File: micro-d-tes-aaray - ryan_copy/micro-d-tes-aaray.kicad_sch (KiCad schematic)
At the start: 46 parts, among them J1 Conn_01x01_Socket, J10 Conn_01x01_Socket, J11 Conn_01x01_Socket, J12 Conn_01x01_Socket, J13 Conn_01x01_Socket, J14 Conn_01x01_Socket, J15 Conn_01x01_Socket, J16 Conn_01x01_Socket, J17 Conn_01x01_Socket, J18 Conn_01x01_Socket, J2 Conn_01x01_Socket, J20 Conn_01x01_Socket, J21 DB25_Plug, J22 Conn_01x01_Socket, J23 Conn_01x01_Socket, J24 Conn_01x01_Socket, J25 Conn_01x01_Socket, J26 Conn_01x01_Socket, J27 Conn_01x01_Socket, J28 Conn_01x01_Socket, J29 Conn_01x01_Socket, J3 Conn_01x01_Socket, J30 Conn_01x01_Socket, J31 Conn_01x01_Socket, J32 Conn_01x01_Socket, J33 Conn_01x01_Socket, J34 Conn_01x01_Socket, J35 Conn_01x01_Socket, J36 Conn_01x01_Socket, J37 Conn_01x01_Socket, J38 Conn_01x01_Socket, J39 Conn_01x01_Socket, J4 Conn_01x01_Socket, J40 Conn_01x01_Socket, J41 Conn_01x01_Socket, J42 DB25_Plug, J5 Conn_01x01_Socket, J6 Conn_01x01_Socket, J7 Conn_01x01_Socket, J8 Conn_01x01_Socket, J9 Conn_01x01_Socket

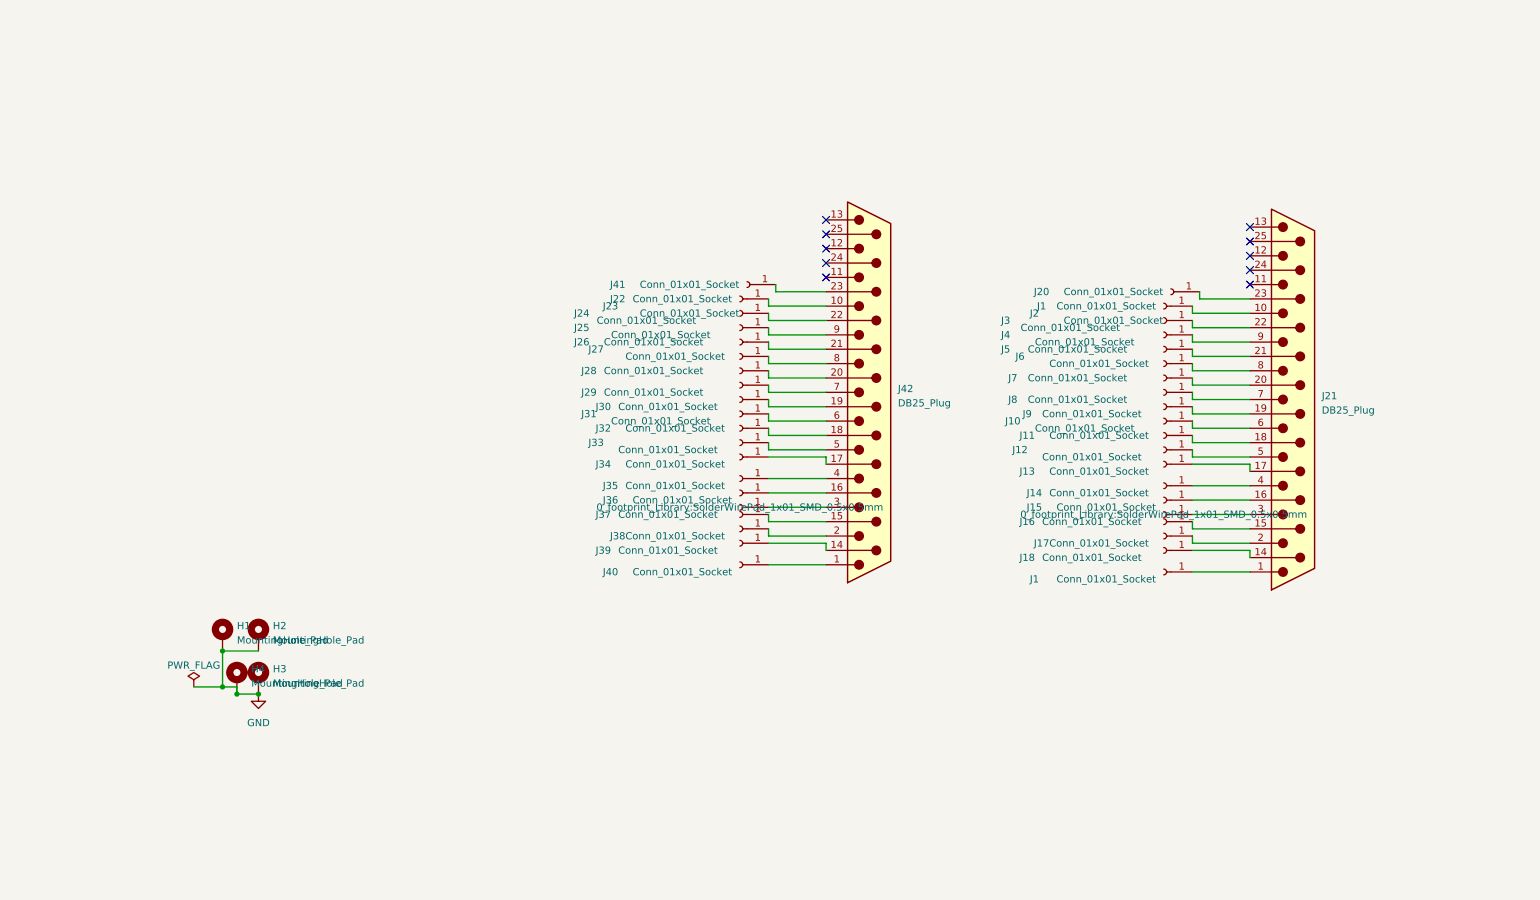
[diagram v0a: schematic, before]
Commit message: update
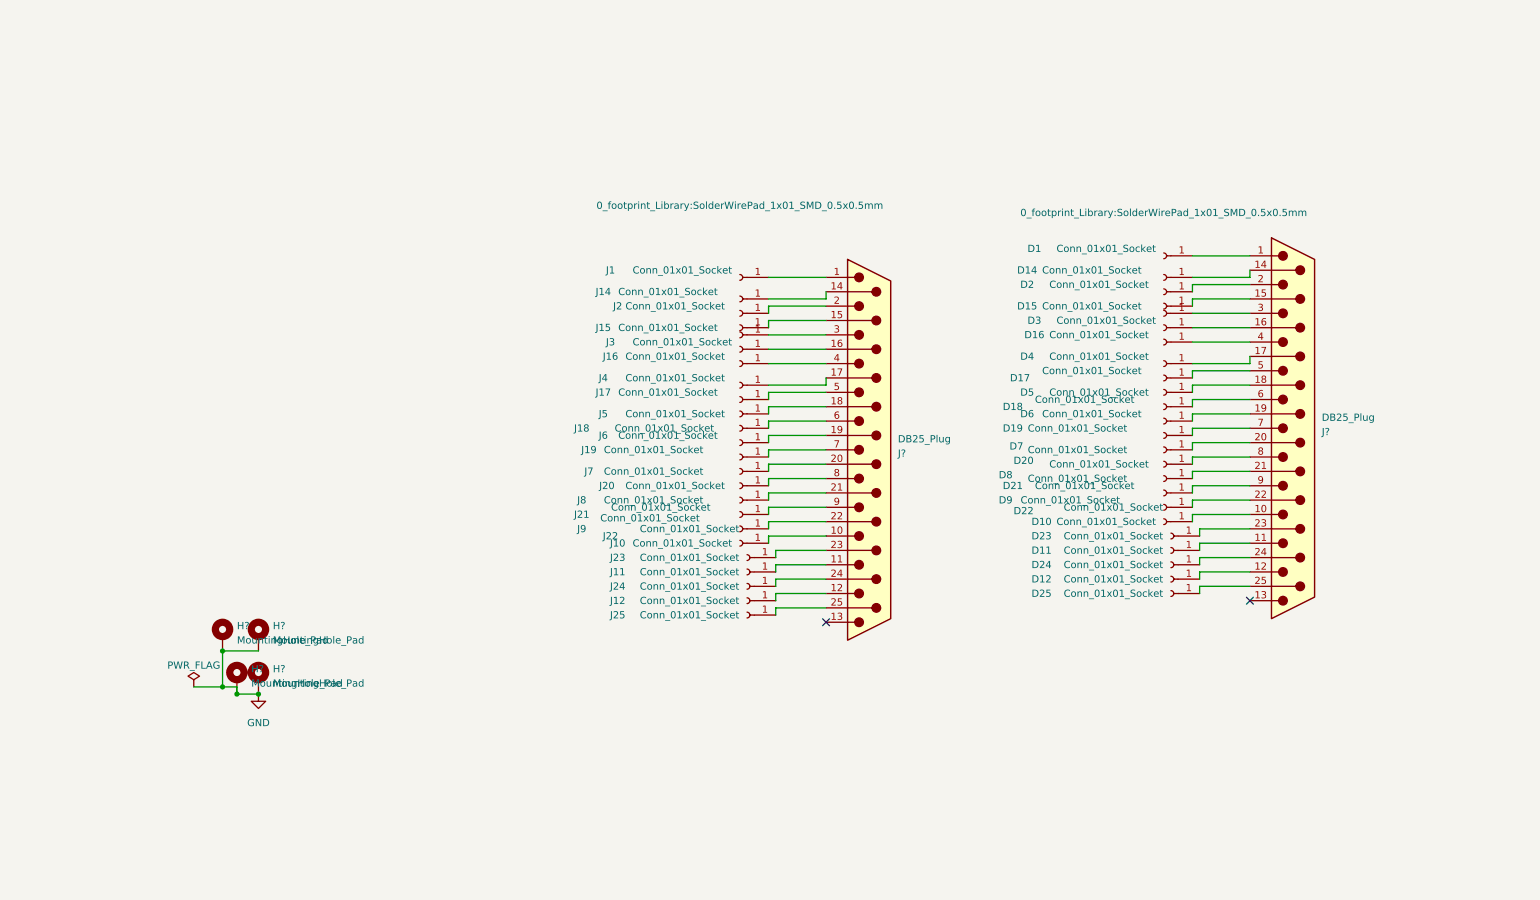
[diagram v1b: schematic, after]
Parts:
- added D11, D12, D24, D25, J11, J12, J24, J25: Conn_01x01_Socket, 0_footprint_Library:SolderWirePad_1x01_SMD_0.5x0.5mm, symbol Connector:Conn_01x01_Socket
- renumbered J1 to D1, J1 to D10, J18 to D14, J16 to D15, J14 to D16, J12 to D17, J10 to D18, J8 to D19, J17 to D2, J6 to D20, J4 to D21, J2 to D22, J20 to D23, J15 to D3, J13 to D4, J11 to D5, J9 to D6, J7 to D7, J5 to D8, J3 to D9, H4 to H?, H1 to H?, H2 to H?, H3 to H?, J40 to J1, J22 to J10, J39 to J14, J37 to J15, J35 to J16, J33 to J17, J31 to J18, J29 to J19, J38 to J2, J27 to J20, J25 to J21, J23 to J22, J41 to J23, J36 to J3, J34 to J4, J32 to J5, J30 to J6, J28 to J7, J26 to J8, J24 to J9, J42 to J?, J21 to J?
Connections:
- net at J?.11: now also J11.1 (Pin_1)
- net at J?.12: now also J12.1 (Pin_1)
- net at J?.24 (P24): now also J24.1 (Pin_1)
- net at J?.25 (P25): now also J25.1 (Pin_1)
- net at J?.11: now also D11.1 (Pin_1)
- net at J?.12: now also D12.1 (Pin_1)
- net at J?.24 (P24): now also D24.1 (Pin_1)
- net at J?.25 (P25): now also D25.1 (Pin_1)
- no-connect marks 10 -> 2
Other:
- moved on the sheet: D1, D10, D14, D15, D16, D17, D18, D19, D2, D20, D21, D22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

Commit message: update pcb
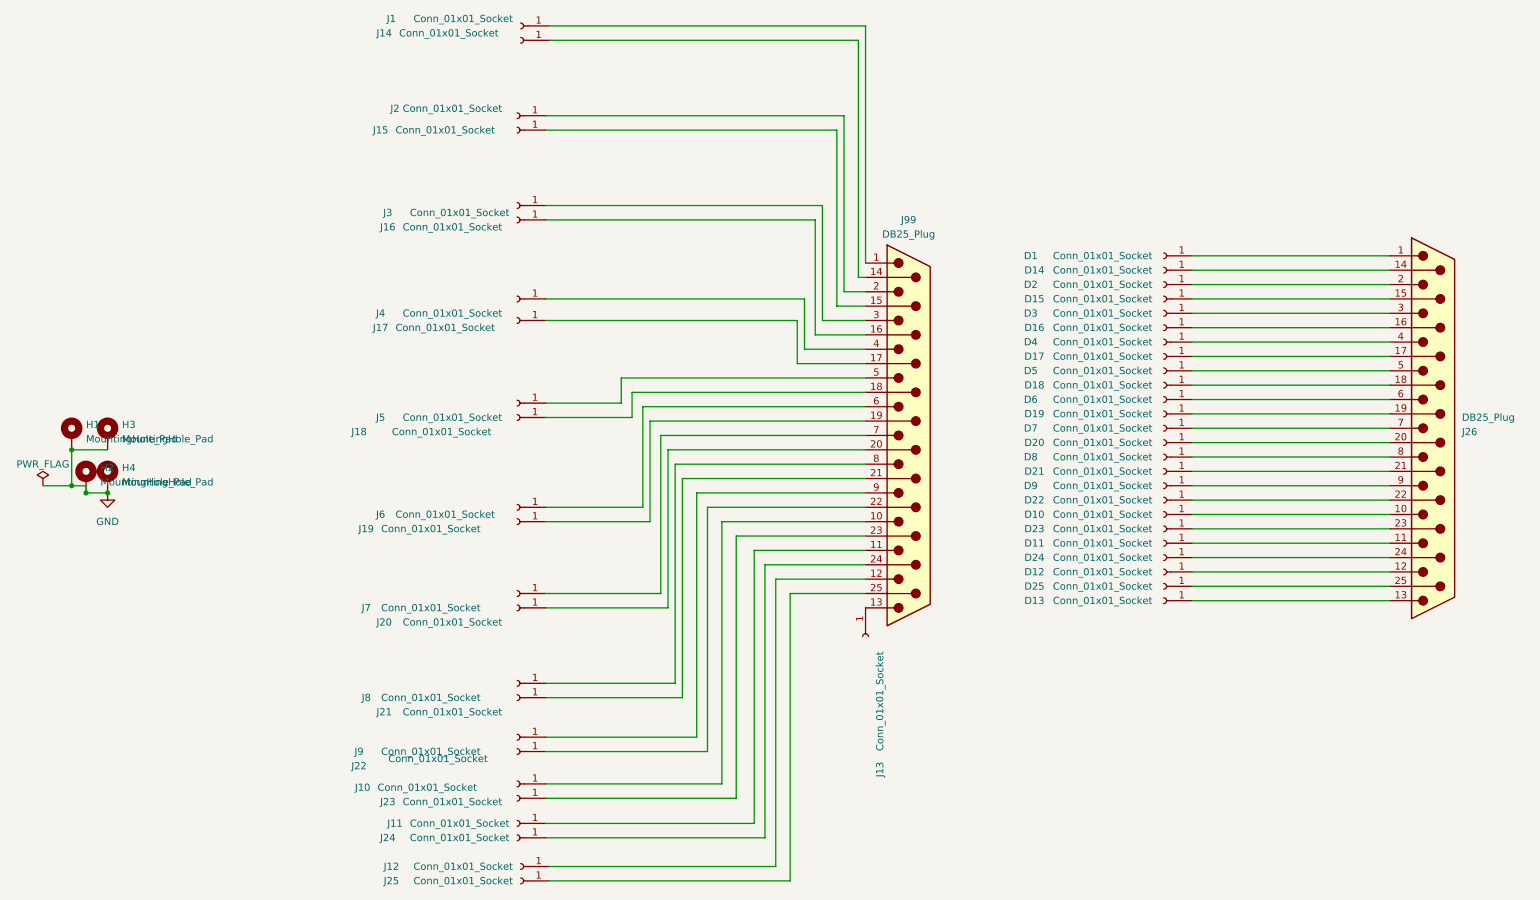
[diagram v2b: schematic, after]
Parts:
- removed J11, J24: Conn_01x01_Socket, 0_footprint_Library:SolderWirePad_1x01_SMD_0.5x0.5mm, symbol Connector:Conn_01x01_Socket
- added D13, J20: Conn_01x01_Socket, 0_footprint_Library:SolderWirePad_1x01_SMD_0.5x2mm_1, symbol Connector:Conn_01x01_Socket
- added J13, J7: Conn_01x01_Socket, 0_footprint_Library:SolderWirePad_1x01_SMD_0.7x2mm, symbol Connector:Conn_01x01_Socket
- D1, D10, D11, D12, D14, D15, D16, D17, D19, D2, D20, D21, D22, D24, D25, D4, D5, D6, D7, D9, J1, J12, J2, J3, J4, J5, J6: footprint 0_footprint_Library:SolderWirePad_1x01_SMD_0.5x0.5mm -> 0_footprint_Library:SolderWirePad_1x01_SMD_0.7x2mm
- D18, D23, D3, D8, J14, J15, J16, J17, J18, J19, J25: footprint 0_footprint_Library:SolderWirePad_1x01_SMD_0.5x0.5mm -> 0_footprint_Library:SolderWirePad_1x01_SMD_0.5x2mm_1
- J10: renamed from J9; footprint 0_footprint_Library:SolderWirePad_1x01_SMD_0.5x0.5mm -> 0_footprint_Library:SolderWirePad_1x01_SMD_0.7x2mm
- J11: renamed from J10; footprint 0_footprint_Library:SolderWirePad_1x01_SMD_0.5x0.5mm -> 0_footprint_Library:SolderWirePad_1x01_SMD_0.7x2mm
- J21: renamed from J20; footprint 0_footprint_Library:SolderWirePad_1x01_SMD_0.5x0.5mm -> 0_footprint_Library:SolderWirePad_1x01_SMD_0.5x2mm_1
- J22: renamed from J21; footprint 0_footprint_Library:SolderWirePad_1x01_SMD_0.5x0.5mm -> 0_footprint_Library:SolderWirePad_1x01_SMD_0.5x2mm_1
- J23: renamed from J22; footprint 0_footprint_Library:SolderWirePad_1x01_SMD_0.5x0.5mm -> 0_footprint_Library:SolderWirePad_1x01_SMD_0.5x2mm_1
- J24: renamed from J23; footprint 0_footprint_Library:SolderWirePad_1x01_SMD_0.5x0.5mm -> 0_footprint_Library:SolderWirePad_1x01_SMD_0.5x2mm_1
- J8: renamed from J7; footprint 0_footprint_Library:SolderWirePad_1x01_SMD_0.5x0.5mm -> 0_footprint_Library:SolderWirePad_1x01_SMD_0.7x2mm
- J9: renamed from J8; footprint 0_footprint_Library:SolderWirePad_1x01_SMD_0.5x0.5mm -> 0_footprint_Library:SolderWirePad_1x01_SMD_0.7x2mm
- gave numbers to parts that had none: 6
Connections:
- net at J99.24 (P24): now also J24.1 (Pin_1)
- net at J9.1 (Pin_1): now also J99.9; no longer J99.8
- net at J23.1 (Pin_1): now also J99.23 (P23); no longer J99.22 (P22)
- net at J22.1 (Pin_1): now also J99.22 (P22); no longer J99.21 (P21)
- net at J21.1 (Pin_1): now also J99.21 (P21); no longer J99.20 (P20)
- net at J11.1 (Pin_1): now also J99.11; no longer J99.10
- net at J8.1 (Pin_1): now also J99.8; no longer J99.7
- net at J10.1 (Pin_1): now also J99.10; no longer J99.9
- net at J99.13: now also J13.1 (Pin_1)
- net at J26.13: now also D13.1 (Pin_1)
- new net: J20.1 (Pin_1), J99.20 (P20)
- new net: J7.1 (Pin_1), J99.7
- no-connect marks 2 -> 0
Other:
- moved on the sheet: D10, D11, D12, D14, D15, D17, D18, D19, D2, D20, D21, D22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
